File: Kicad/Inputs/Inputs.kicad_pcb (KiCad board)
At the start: 2 copper layers, 5 parts

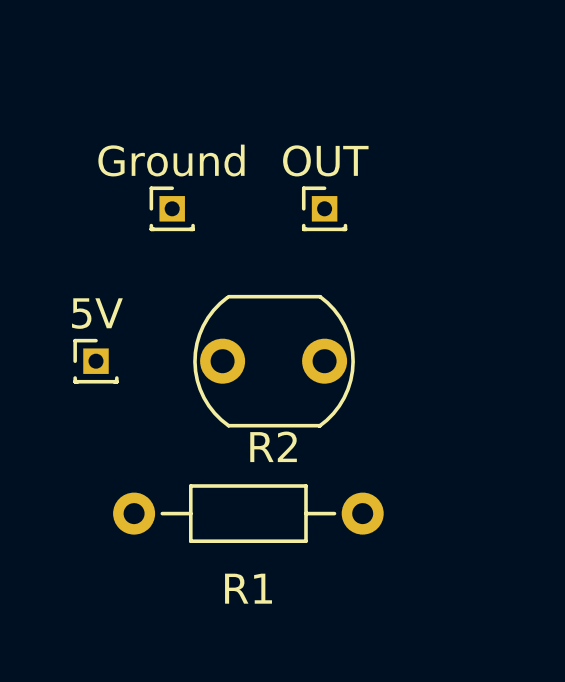
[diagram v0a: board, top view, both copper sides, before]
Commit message: Update
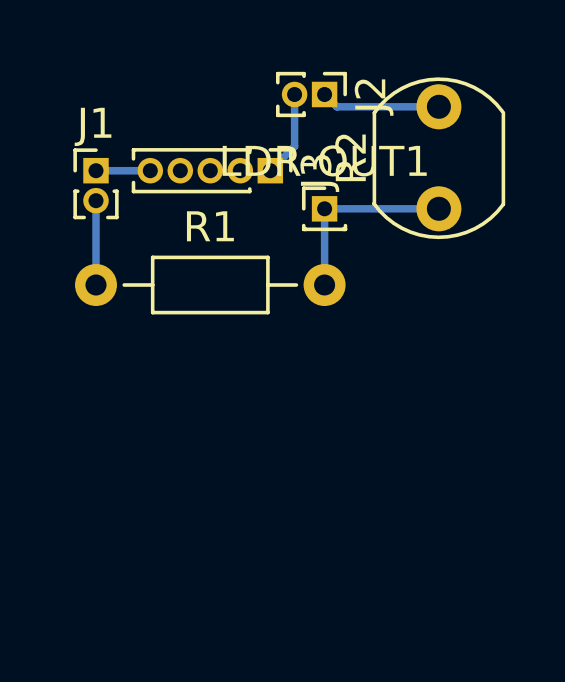
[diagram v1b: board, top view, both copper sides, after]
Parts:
- removed 5V: 5V, Connector_PinHeader_1.00mm:PinHeader_1x01_P1.00mm_Vertical
- removed Ground: Ground, Connector_PinHeader_1.00mm:PinHeader_1x01_P1.00mm_Vertical
- removed OUT: OUT, Connector_PinHeader_1.00mm:PinHeader_1x01_P1.00mm_Vertical
- added J1: 5V, Connector_PinHeader_1.00mm:PinHeader_1x02_P1.00mm_Vertical, F.Cu at (134.6, 82.5)
- added J2: GROUND, Connector_PinHeader_1.00mm:PinHeader_1x02_P1.00mm_Vertical, F.Cu at (142.2, 80.0)
- added J3: Conn_01x05_Female, Connector_PinHeader_1.00mm:PinHeader_1x05_P1.00mm_Vertical, F.Cu at (140.4, 82.5)
- added LDR-OUT1: LDR-OUT, Connector_PinHeader_1.00mm:PinHeader_1x01_P1.00mm_Vertical, F.Cu at (142.2, 83.8)
- moved R1 7.73 mm to (134.6, 86.4)
- moved R2 6.35 mm to (146.1, 83.8), turned to 90 degrees
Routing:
- net Net-(LDR-OUT1-Pad1): track 0.00 -> 6.35 mm
- net Net-(R2-Pad2): track 0.00 -> 3.98 mm
- net Net-(J2-Pad2): track 0.00 -> 2.88 mm
- net Net-(R1-Pad1): track 0.00 -> 2.81 mm
- net Net-(J1-Pad1): track 0.00 -> 1.81 mm
